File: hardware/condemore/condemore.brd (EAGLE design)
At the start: 86 x 56 mm, 4 parts

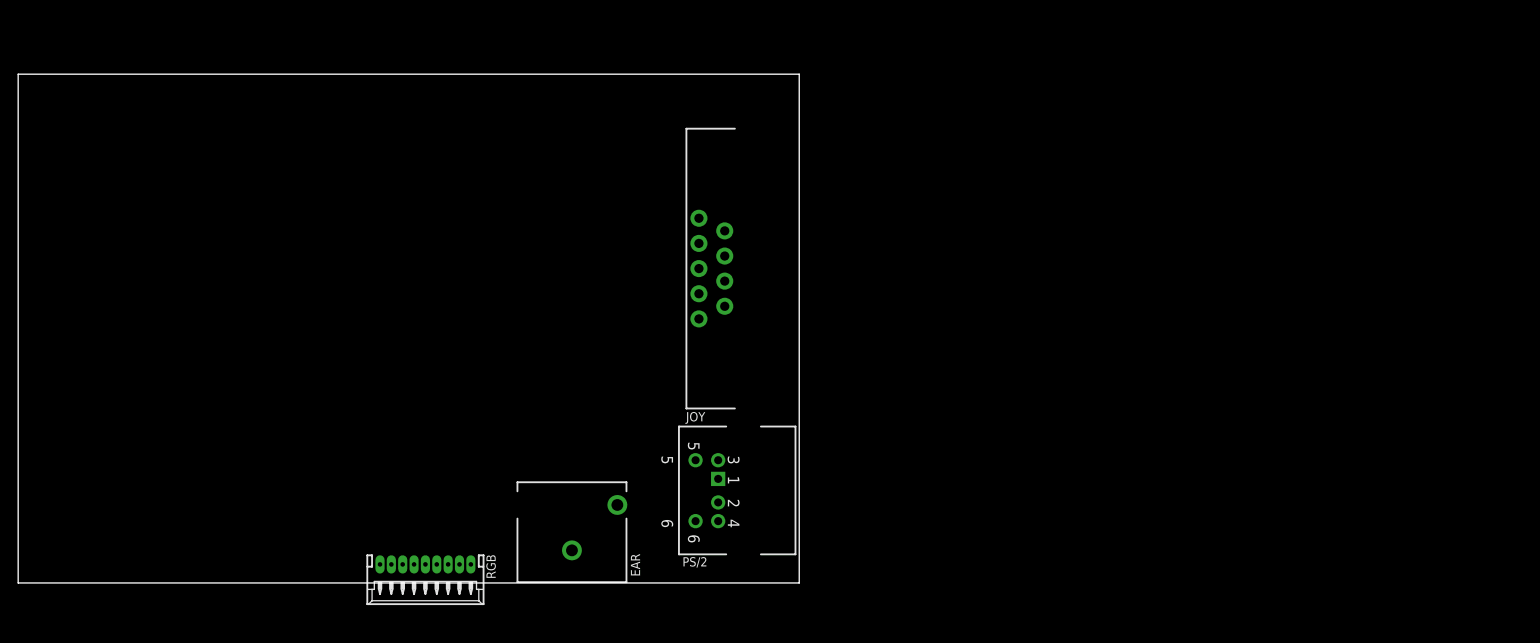
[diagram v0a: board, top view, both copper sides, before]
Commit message: Actualizo condemore
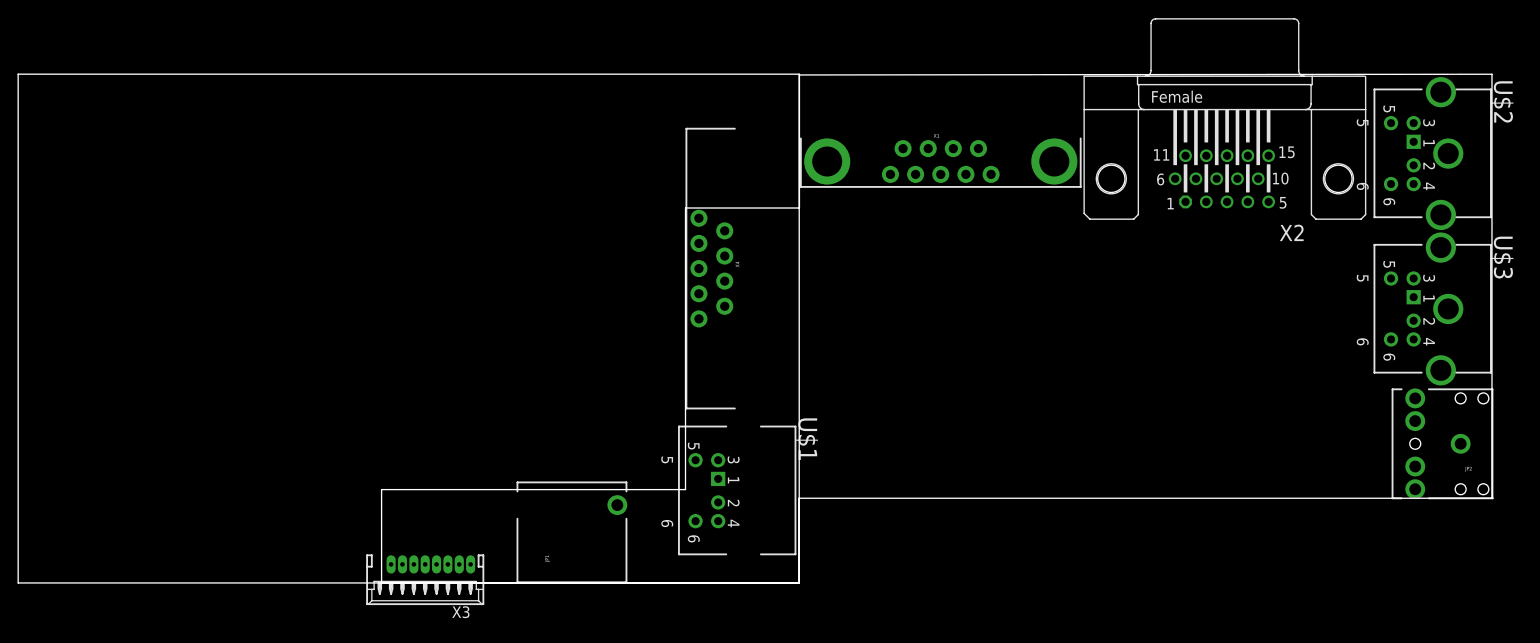
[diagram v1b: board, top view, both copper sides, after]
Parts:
- removed EAR: EAR, SparkFun-Connectors:AUDIO-JACK
- removed JOY: (no value), SparkFun-Connectors:DB9_MALE
- removed PS/2: PS/2 Keyb, ZX_UNO_0_14:DINC/MIN_TM/6_1PRIMARY
- removed RGB: RGB, con-molex:53048-09
- added JP1: (no value), SparkFun-Connectors_huella:AUDIO-JACK_HUELLA
- added JP2: (no value), SparkFun-Connectors:AUDIO-JACK
- added U$1: DINC_MINI_HUELLA, ZX_UNO_0_14_huella:DINC/MIN_TM/6_1PRIMARY_HUELLA
- added U$2, U$3: DINC_MIN_TM_6_1, ZX_UNO_0_14:DINC/MIN_TM/6_1PRIMARY
- added X1: (no value), SparkFun-Connectors:DB9_MALE
- added X2: (no value), con-subd:HDF15H
- added X3: 53048-09_HUELLA, con-molex_huella:53048-09_HUELLA
- added X4: (no value), SparkFun-Connectors_huella:DB9_MALE
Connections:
- net 3.3V: now also X3.4; no longer RGB.4
- net 5V: now also U$1.4; no longer PS/2.4
- net B: now also X3.7; no longer RGB.7
- net CSYNC: now also X3.3; no longer RGB.3
- net G: now also X3.6; no longer RGB.6
- net GND: now also U$1.3, X4.8; no longer JOY.8, PS/2.3, RGB.1
- net JOY_FIRE1: now also X4.6; no longer JOY.6
- net JOY_FIRE2: now also X4.9; no longer JOY.9
- net JOY_LEFT: now also X4.3; no longer JOY.3
- net JOY_RIGHT: now also X4.4; no longer JOY.4
- net L-OUT: now also X3.9; no longer RGB.9
- net N$1: now also U$1.6; no longer PS/2.6
- net N$2: now also U$1.5; no longer PS/2.5
- net N$3: now also U$1.2; no longer PS/2.2
- net N$4: now also U$1.1; no longer PS/2.1
- net PIN5: now also X4.5; no longer JOY.5
- net PIN7: now also X4.7; no longer JOY.7
- net R: now also X3.5; no longer RGB.5
- net R-OUT: now also X3.8; no longer RGB.8
- net VSYNC: now also X3.2; no longer RGB.2
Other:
- board size 86 x 56 mm -> 162.4 x 56 mm
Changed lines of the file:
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@@
 <layer number="44" name="Drills" color="7" fill="1" visible="no" active="yes"/>
 <layer number="45" name="Holes" color="7" fill="1" visible="no" active="yes"/>
-<layer number="46" name="Milling" color="3" fill="1" visible="no" active="yes"/>
+<layer number="46" name="Milling" color="3" fill="1" visible="yes" active="yes"/>
 <layer number="47" name="Measures" color="7" fill="1" visible="no" active="yes"/>
 <layer number="48" name="Document" color="7" fill="1" visible="no" active="yes"/>
@@
 <text x="6.4285875" y="0.63690625" size="1.016" layer="125" font="vector" ratio="15">Y1</text>
 <text x="21.719640625" y="0.5897625" size="1.016" layer="125" font="vector" ratio="15">Y2</text>
+<wire x1="40.005" y1="10.2790625" x2="40.005" y2="0" width="0" layer="46"/>
+<wire x1="162.236875" y1="9.286875" x2="162.236875" y2="56" width="0" layer="46"/>
+<wire x1="162.236875" y1="56" x2="86.0028125" y2="55.920625" width="0" layer="46"/>
+<wire x1="73.3821875" y1="10.2790625" x2="40.005" y2="10.2790625" width="0" layer="46"/>
+<wire x1="40.005" y1="0" x2="85.963125" y2="0" width="0" layer="46"/>
+<wire x1="85.963125" y1="0" x2="85.963125" y2="9.3265625" width="0" layer="46"/>
+<wire x1="85.963125" y1="9.3265625" x2="162.3615625" y2="9.3265625" width="0" layer="46"/>
+<wire x1="73.421875" y1="10.2790625" x2="73.4615625" y2="10.2790625" width="0" layer="46"/>
+<wire x1="73.4615625" y1="10.2790625" x2="73.4615625" y2="41.275" width="0" layer="46"/>
+<wire x1="73.4615625" y1="41.275" x2="86.0028125" y2="41.275" width="0" layer="46"/>
+<wire x1="86.0028125" y1="41.275" x2="86.0028125" y2="55.9196875" width="0" layer="46"/>
 </plain>
 <attributes>
@@
 </autorouter>
 <elements>
-<element name="EAR" library="SparkFun-Connectors" package="AUDIO-JACK" value="EAR" x="60.96" y="3.58775" smashed="yes" rot="R90">
-<attribute name="NAME" x="67.447771875" y="3.22800625" size="1.016" layer="25" font="vector" ratio="15" rot="R270"/>
-<attribute name="VALUE" x="59.69" y="2.31775" size="0.4064" layer="27" rot="R90"/>
+<element name="X2" library="con-subd" package="HDF15H" value="" x="132.8340625" y="44.4896875" rot="R180">
+<attribute name="OC_FARNELL" value="unknown" x="132.8340625" y="44.4896875" size="1.778" layer="27" rot="R180" display="off"/>
+<attribute name="MF" value="" x="132.8340625" y="44.4896875" size="1.778" layer="27" rot="R180" display="off"/>
+<attribute name="OC_NEWARK" value="unknown" x="132.8340625" y="44.4896875" size="1.778" layer="27" rot="R180" display="off"/>
+<attribute name="MPN" value="" x="132.8340625" y="44.4896875" size="1.778" layer="27" rot="R180" display="off"/>
 </element>
-<element name="JOY" library="SparkFun-Connectors" package="DB9_MALE" value="" x="76.35875" y="34.6075" smashed="yes" rot="R270">
-<attribute name="NAME" x="73.5127875" y="17.79186875" size="1.016" layer="25" font="vector" ratio="15"/>
-<attribute name="VALUE" x="79.77375" y="35.2975" size="0.4064" layer="27" ratio="10" rot="R270"/>
+<element name="U$1" library="ZX_UNO_0_14_huella" package="DINC/MIN_TM/6_1PRIMARY_HUELLA" value="DINC_MINI_HUELLA" x="85.56625" y="10.16" rot="R270"/>
+<element name="U$2" library="ZX_UNO_0_14" package="DINC/MIN_TM/6_1PRIMARY" value="DINC_MIN_TM_6_1" x="162.1234375" y="47.2678125" rot="R270"/>
+<element name="U$3" library="ZX_UNO_0_14" package="DINC/MIN_TM/6_1PRIMARY" value="DINC_MIN_TM_6_1" x="162.1234375" y="30.1625" rot="R270"/>
+<element name="X3" library="con-molex_huella" package="53048-09_HUELLA" value="53048-09_HUELLA" x="44.8071875" y="0.79375" rot="R180">
+<attribute name="OC_FARNELL" value="1012239" x="44.8071875" y="0.79375" size="1.778" layer="27" rot="R180" display="off"/>
+<attribute name="MF" value="" x="44.8071875" y="0.79375" size="1.778" layer="27" rot="R180" display="off"/>
+<attribute name="OC_NEWARK" value="98K9837" x="44.8071875" y="0.79375" size="1.778" layer="27" rot="R180" display="off"/>
+<attribute name="MPN" value="53048-0910" x="44.8071875" y="0.79375" size="1.778" layer="27" rot="R180" display="off"/>
 </element>
-<element name="RGB" library="con-molex" package="53048-09" value="RGB" x="44.831" y="0.79375" smashed="yes" rot="R180">
-<attribute name="OC_NEWARK" value="98K9837" x="44.831" y="0.79375" size="1.778" layer="27" rot="R180" display="off"/>
-<attribute name="MPN" value="53048-0910" x="44.831" y="0.79375" size="1.778" layer="27" rot="R180" display="off"/>
-<attribute name="MF" value="" x="44.831" y="0.79375" size="1.778" layer="27" rot="R180" display="off"/>
-<attribute name="OC_FARNELL" value="1012239" x="44.831" y="0.79375" size="1.778" layer="27" rot="R180" display="off"/>
-<attribute name="NAME" x="51.5493875" y="3.143325" size="1.016" layer="25" font="vector" ratio="15" rot="R270"/>
-<attribute name="VALUE" x="50.831" y="4.54375" size="1.27" layer="27" rot="R180"/>
-</element>
-<element name="PS/2" library="ZX_UNO_0_14" package="DINC/MIN_TM/6_1PRIMARY" value="PS/2 Keyb" x="85.56625" y="10.16" smashed="yes" rot="R270">
-<attribute name="NAME" x="73.115196875" y="1.818396875" size="1.016" layer="25" font="vector" ratio="15" rot="SR0"/>
-<attribute name="VALUE" x="85.66785" y="18.3388" size="2.032" layer="27" font="vector" ratio="13" rot="SR270"/>
-</element>
+<element name="JP1" library="SparkFun-Connectors_huella" package="AUDIO-JACK_HUELLA" value="" x="60.96" y="3.571875" rot="R90"/>
+<element name="X4" library="SparkFun-Connectors_huella" package="DB9_MALE" value="" x="76.35875" y="34.6075" rot="R270"/>
+<element name="X1" library="SparkFun-Connectors" package="DB9_MALE" value="" x="101.5603125" y="46.3946875"/>
+<element name="JP2" library="SparkFun-Connectors" package="AUDIO-JACK" value="" x="158.7896875" y="15.319375" rot="R180"/>
 </elements>
 <signals>
 <signal name="GND">
-<contactref element="JOY" pad="8"/>
-<contactref element="PS/2" pad="3"/>
-<contactref element="RGB" pad="1"/>
+<contactref element="U$1" pad="3"/>
+<contactref element="X4" pad="8"/>
 <wire x1="77.05725" y1="13.5128" x2="77.77875" y2="35.9875" width="0" layer="19" extent="1-1"/>
-<wire x1="39.831" y1="2.04375" x2="77.05725" y2="13.5128" width="0" layer="19" extent="1-1"/>
+</signal>
+<signal name="N$1">
+<contactref element="U$1" pad="6"/>
+</signal>
+<signal name="N$2">
+<contactref element="U$1" pad="5"/>
+</signal>
+<signal name="N$3">
+<contactref element="U$1" pad="2"/>
+</signal>
+<signal name="N$4">
+<contactref element="U$1" pad="1"/>
+</signal>
+<signal name="5V">
+<contactref element="U$1" pad="4"/>
+</signal>
+<signal name="VSYNC">
+<contactref element="X3" pad="2"/>
+</signal>
+<signal name="CSYNC">
+<contactref element="X3" pad="3"/>
 </signal>
 <signal name="3.3V">
-<contactref element="RGB" pad="4"/>
-</signal>
-<signal name="VSYNC">
-<contactref element="RGB" pad="2"/>
-</signal>
-<signal name="CSYNC">
-<contactref element="RGB" pad="3"/>
-</signal>
-<signal name="N$1">
-<contactref element="PS/2" pad="6"/>
-</signal>
-<signal name="N$2">
-<contactref element="PS/2" pad="5"/>
-</signal>
-<signal name="N$3">
-<contactref element="PS/2" pad="2"/>
-</signal>
-<signal name="N$4">
-<contactref element="PS/2" pad="1"/>
+<contactref element="X3" pad="4"/>
 </signal>
 <signal name="R">
-<contactref element="RGB" pad="5"/>
+<contactref element="X3" pad="5"/>
+</signal>
+<signal name="G">
+<contactref element="X3" pad="6"/>
 </signal>
 <signal name="B">
-<contactref element="RGB" pad="7"/>
+<contactref element="X3" pad="7"/>
 </signal>
 <signal name="R-OUT">
-<contactref element="RGB" pad="8"/>
+<contactref element="X3" pad="8"/>
 </signal>
 <signal name="L-OUT">
-<contactref element="RGB" pad="9"/>
-</signal>
-<signal name="5V">
-<contactref element="PS/2" pad="4"/>
-</signal>
-<signal name="G">
-<contactref element="RGB" pad="6"/>
+<contactref element="X3" pad="9"/>
 </signal>
 <signal name="JOY_LEFT">
-<contactref element="JOY" pad="3"/>
+<contactref element="X4" pad="3"/>
 </signal>
 <signal name="JOY_RIGHT">
-<contactref element="JOY" pad="4"/>
+<contactref element="X4" pad="4"/>
 </signal>
 <signal name="JOY_FIRE1">
-<contactref element="JOY" pad="6"/>
+<contactref element="X4" pad="6"/>
 </signal>
 <signal name="JOY_FIRE2">
-<contactref element="JOY" pad="9"/>
+<contactref element="X4" pad="9"/>
 </signal>
 <signal name="PIN7">
-<contactref element="JOY" pad="7"/>
+<contactref element="X4" pad="7"/>
 </signal>
 <signal name="PIN5">
-<contactref element="JOY" pad="5"/>
+<contactref element="X4" pad="5"/>
 </signal>
 </signals>
